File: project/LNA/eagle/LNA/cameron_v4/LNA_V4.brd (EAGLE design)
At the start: 36 x 26.4 mm, 18 parts, among them Q1 MMBT3906LT1SMD, Q2 MMBT3906LT1SMD, Q3 SAV-541+, X1 PROBE_LANDING, X2 PROBE_LANDING, X3 332-02

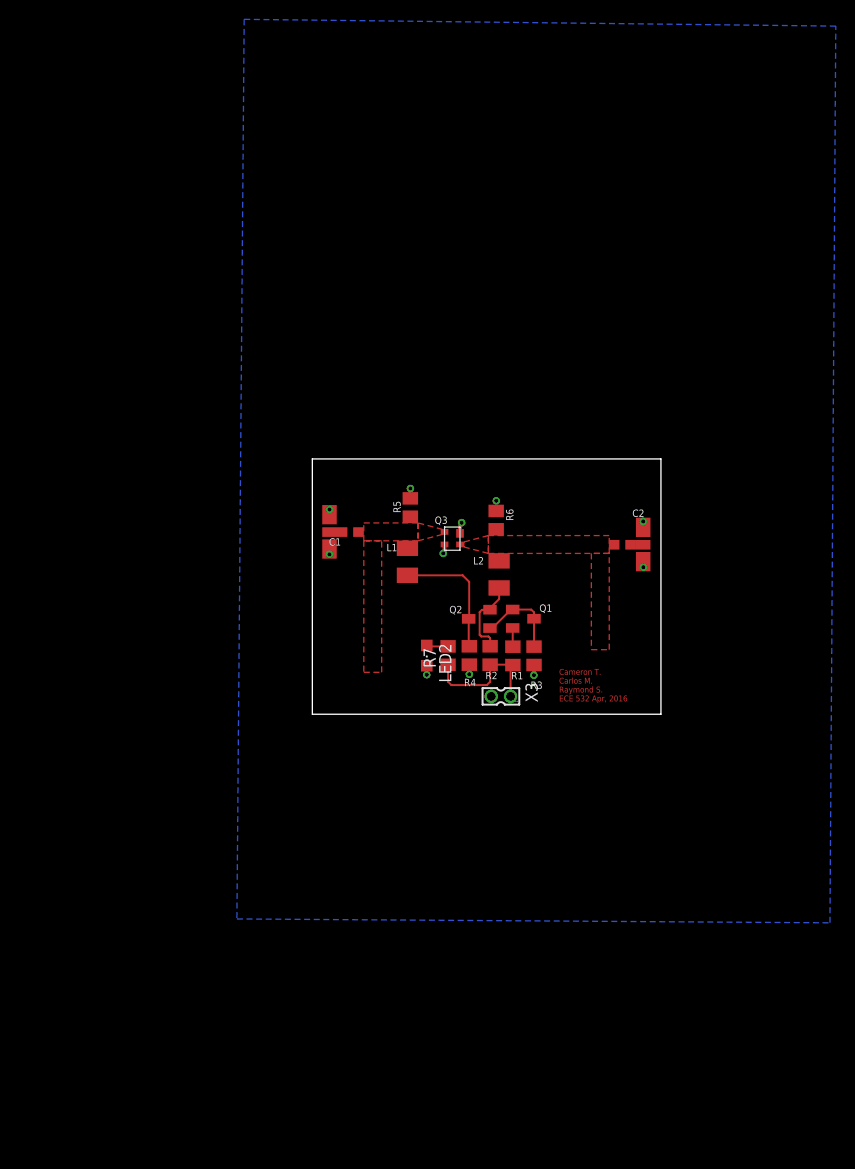
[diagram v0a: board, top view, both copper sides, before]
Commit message: created gerbers for version 4 LNA
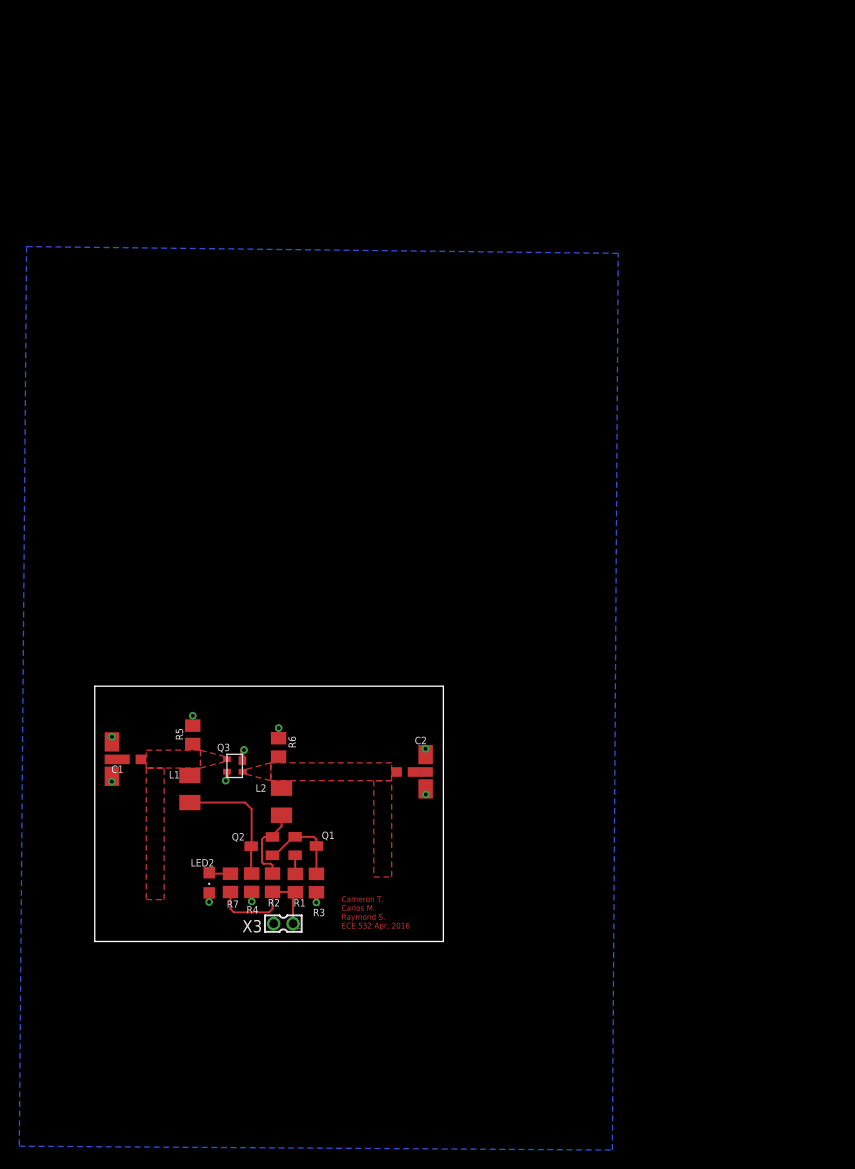
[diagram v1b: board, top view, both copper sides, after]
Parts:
- moved C1 32.5 mm to (3.87, 19.1)
- moved C2 32.5 mm to (32.0, 17.8)
- moved L1 32.5 mm to (9.78, 16.1)
- moved L2 32.5 mm to (19.3, 14.8)
- moved LED2 32.5 mm to (11.8, 6.36)
- moved Q1 32.5 mm to (21.8, 10.2)
- moved Q2 32.5 mm to (17.2, 10.2)
- moved Q3 32.5 mm to (13.6, 19.2)
- moved R1 32.5 mm to (20.7, 6.34)
- moved R2 32.5 mm to (18.3, 6.37)
- moved R3 32.5 mm to (22.9, 6.34)
- moved R4 32.5 mm to (16.2, 6.37)
- moved R5 32.5 mm to (10.1, 21.7)
- moved R6 32.5 mm to (19.0, 20.4)
- moved R7 32.5 mm to (14.0, 6.36)
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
